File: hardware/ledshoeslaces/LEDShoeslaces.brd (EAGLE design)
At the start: 50 x 38 mm, 13 parts, among them IC1 LM1117MPX-5.0

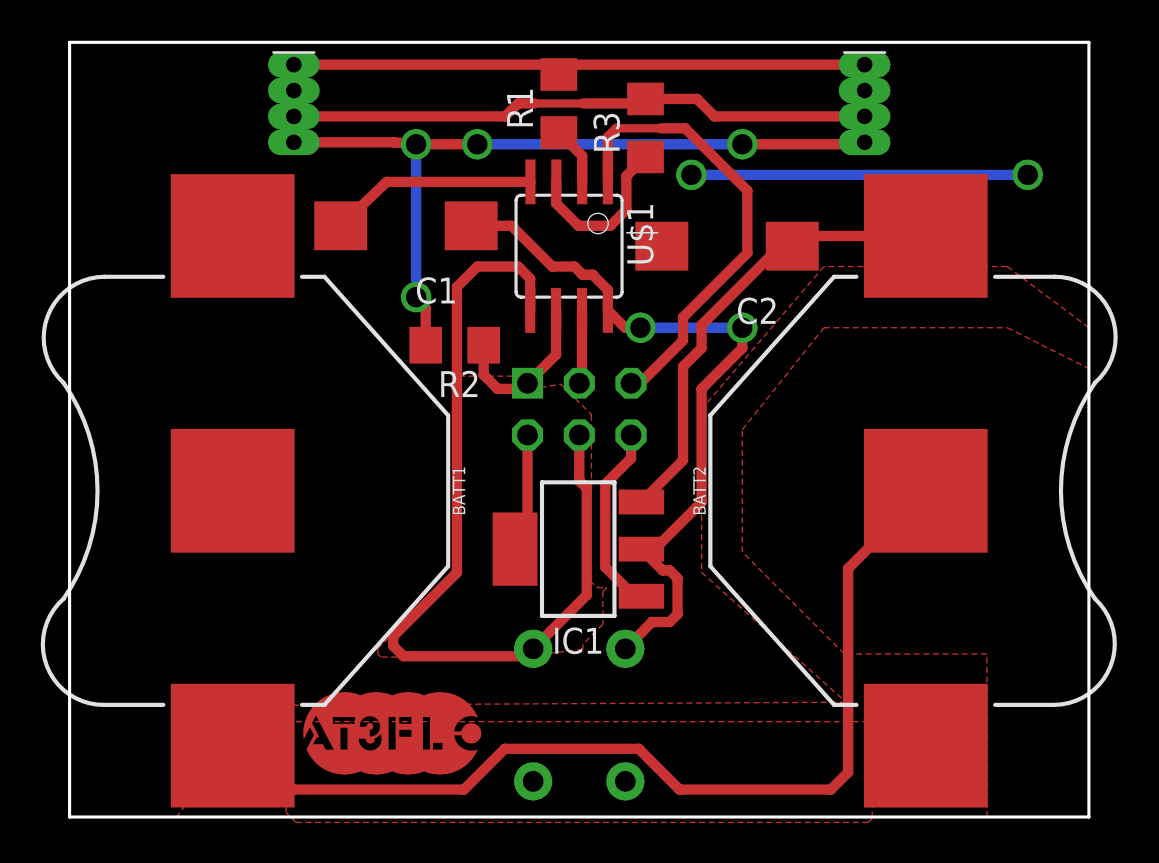
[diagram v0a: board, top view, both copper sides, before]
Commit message: fix spacings
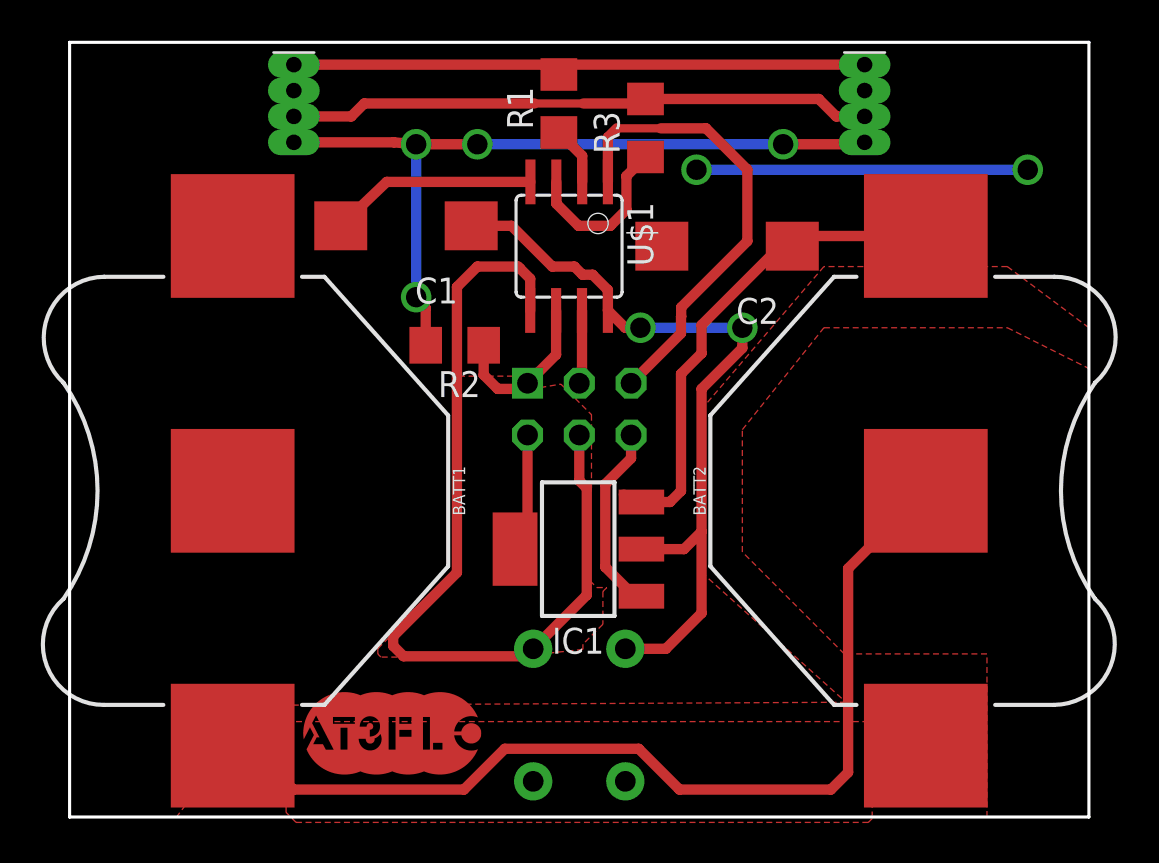
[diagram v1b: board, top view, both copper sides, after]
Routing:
- net VCC: track 42.5 -> 44.4 mm
- net V_BATT: track 24.7 -> 25.5 mm
